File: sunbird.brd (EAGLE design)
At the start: 127 x 19.1 mm, 41 parts, among them J1 USB_MINI-B_SMT, Q1 600mA/40V, U1000 TP4056, U1500 FS312F-G, U1550 FS8205, U2000 MT3608, U4000 FM116B, U5000 CH340G, Y5000 12Mhz

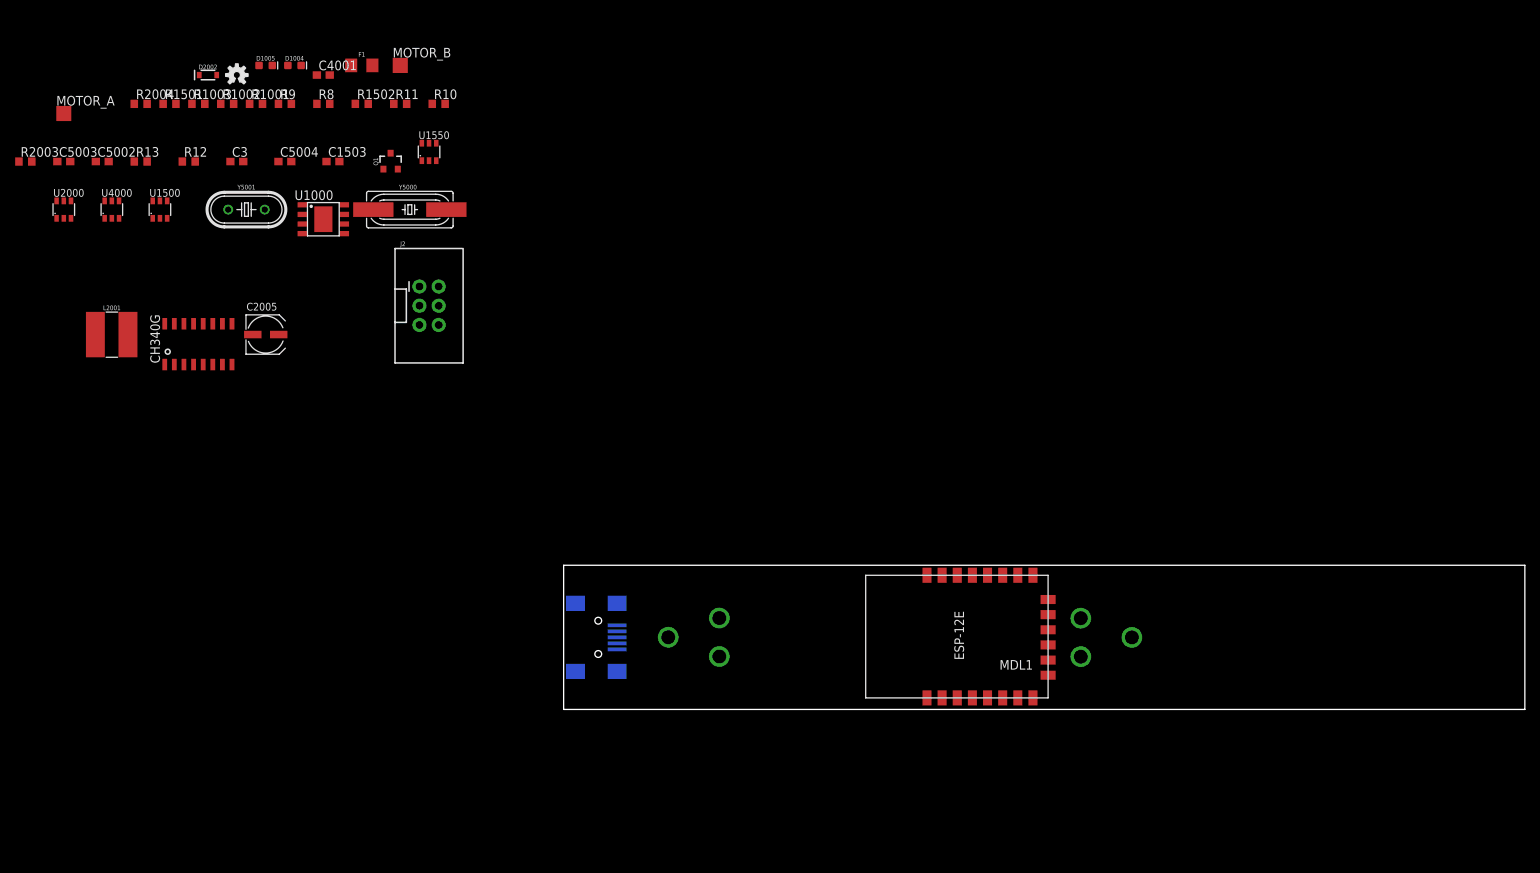
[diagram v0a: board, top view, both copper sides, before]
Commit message: Getting there
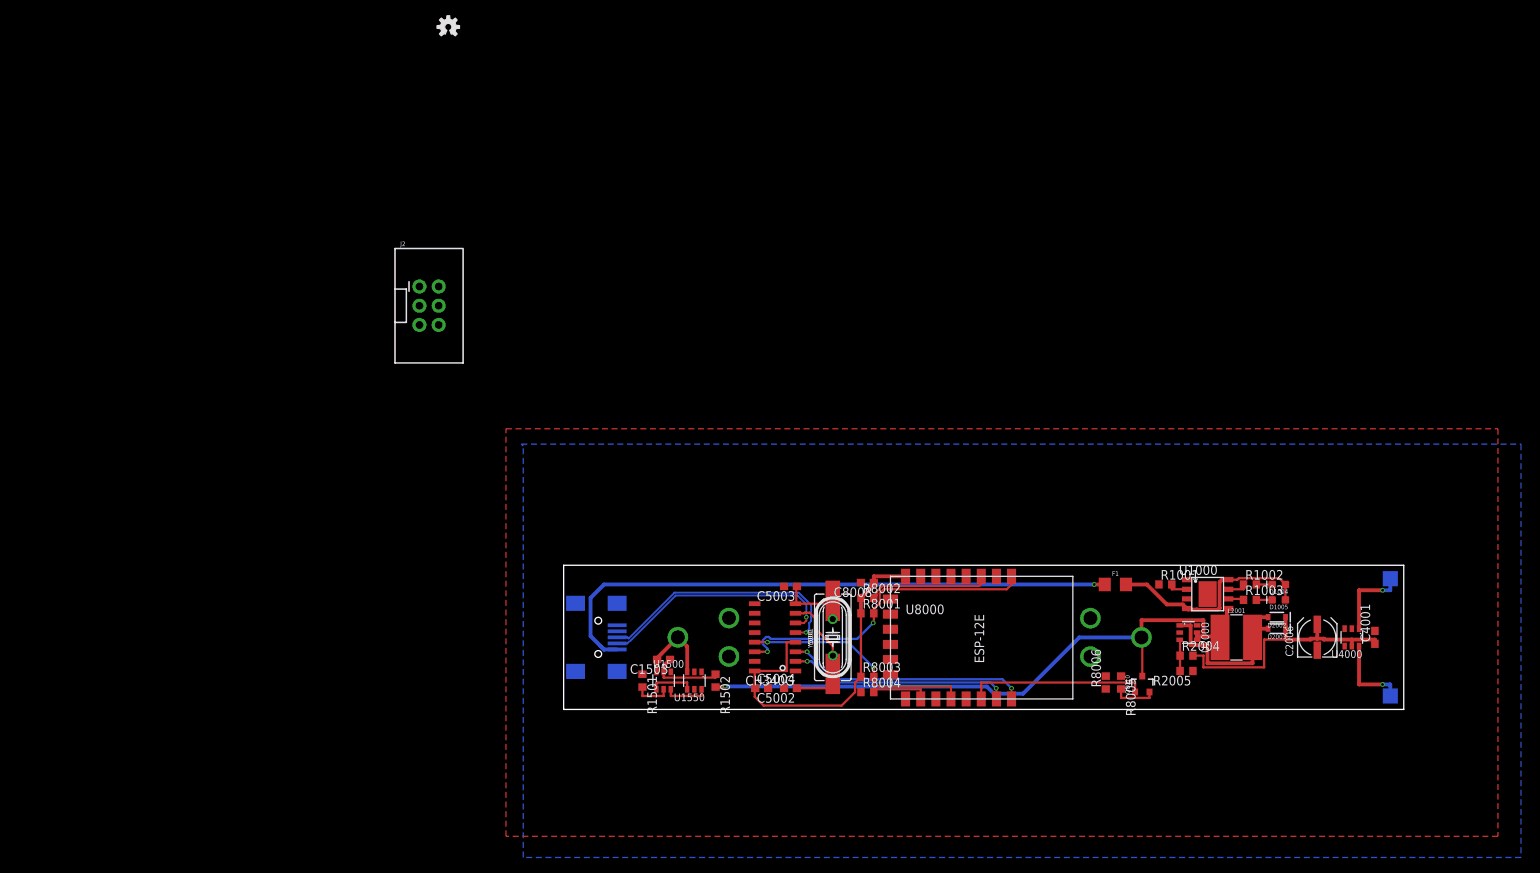
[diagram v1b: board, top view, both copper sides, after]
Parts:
- removed C2005: 47uF, rcl:UD-5X5,8_NICHICON
- removed C3: 0.1uf, rcl:C0603
- removed MDL1: (no value), ESP8266-ESP12E:ESP8266-ESP12E
- removed Q1: 600mA/40V, SparkFun-DiscreteSemi:SOT23-3
- removed R10, R11, R8, R9: 10k, rcl:R0603
- removed R12: 400k, rcl:R0603
- removed R13: 100k, rcl:R0603
- removed R2003: 4.5k, rcl:R0603
- added C2006: 47uF, rcl:UD-5X5,8_NICHICON
- added C8008: 0.1uf, rcl:C0603
- added D2003: (no value), SparkFun-DiscreteSemi:SOD-323
- added Q8010: 600mA/40V, SparkFun-DiscreteSemi:SOT23-3
- added R2005: 1k, rcl:R0603
- added R8001, R8002, R8003, R8004: 10k, rcl:R0603
- added R8005: 400k, rcl:R0603
- added R8006: 100k, rcl:R0603
- added U8000: (no value), ESP8266-ESP12E:ESP8266-ESP12E
- R2004: value 1k -> 4.5k
- moved MOTOR_A 191.4 mm to (109.2, 1.78), flipped to the bottom
- moved U4000 173.3 mm to (104.1, 9.53), turned to 180 degrees
- moved U2000 158.8 mm to (82.5, 10.2), turned to 270 degrees
- moved D2002 158.4 mm to (94.2, 12.2), turned to 180 degrees
- moved C4001 157.6 mm to (107.2, 9.53), turned to 90 degrees
- moved R2004 156.2 mm to (82.3, 7.11)
- moved L2001 153.9 mm to (88.9, 9.53)
- moved R1003 153.6 mm to (90.7, 14.5)
- moved D1005 151.3 mm to (94.5, 14.5), turned to 180 degrees
- moved R1002 149.3 mm to (90.7, 16.5)
- moved MOTOR_B 147.3 mm to (109.2, 17.3), flipped to the bottom
- moved D1004 147.0 mm to (94.5, 16.5), turned to 180 degrees
- moved R1001 135.9 mm to (79.5, 16.5)
- moved U1000 126.9 mm to (85.1, 15.2)
- moved F1 120.9 mm to (72.9, 16.5)
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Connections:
- net N$14 renamed MOTOR_A
- net N$15 renamed MOTOR_B
- removed net SCL: MDL1.14
- removed net SDA: MDL1.13
- removed net USB_D+: U5000.5
- removed net USB_D-: U5000.6
- new net GPIO4: U8000.13
- new net GPIO5: Q8010.1, U8000.14
- net 3.3V: now also C2006.+, C8008.1, D2003.C, R2004.2, R8001.1, R8002.1, R8003.1, U8000.8; no longer C2005.+, C3.1, MDL1.8, R10.1, R2003.2, R8.1, R9.1
- net ADC: now also R8005.1, R8006.2, U8000.2; no longer MDL1.2, R12.1, R13.2
- net CH_PD: now also R8002.2, U8000.3; no longer MDL1.3, R9.2
- net CS0: now also U8000.17; no longer MDL1.17
- net GND: now also C2006.-, C8008.2, R2005.1, R8004.1, R8006.1, U8000.9; no longer C2005.-, C3.2, MDL1.9, R11.1, R13.1, R2004.1
- net GPIO0: now also R8003.2, U8000.12; no longer MDL1.12, R10.2
- net GPIO10: now also U8000.20; no longer MDL1.20
- net GPIO12: now also U8000.6; no longer MDL1.6
- net GPIO13: now also U8000.7; no longer MDL1.7
- net GPIO14: now also U8000.5; no longer MDL1.5
- net GPIO15: now also R8004.2, U8000.10; no longer MDL1.10, R11.2
- net GPIO16: now also U8000.4; no longer MDL1.4, Q1.1
- net GPIO2: now also U8000.11; no longer MDL1.11
- net GPIO9: now also U8000.19; no longer MDL1.19
- net MISO: now also U8000.18; no longer MDL1.18
- net MOSI: now also U8000.21; no longer MDL1.21
- net N$12: now also D2003.A
- net N$13: now also R2004.1, R2005.2; no longer R2003.1, R2004.2
- net N$9: now also Q8010.2, R8005.2; no longer Q1.2, R12.2
- net RESET: now also R8001.2, U8000.1; no longer MDL1.1, R8.2
- net RX: now also U8000.15; no longer MDL1.15
- net SCLK: now also U8000.22; no longer MDL1.22
- net TX: now also U8000.16; no longer MDL1.16
- net USB_N: now also U5000.6
- net USB_P: now also U5000.5
- net V_BATT: now also Q8010.3; no longer Q1.3
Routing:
- net V_BATT: track 0.00 -> 86.6 mm, vias 0 -> 1
- net 3.3V: track 0.00 -> 83.5 mm
- net N$17: track 0.00 -> 78.7 mm, vias 0 -> 1
- net RESET: track 0.00 -> 42.4 mm, vias 0 -> 2
- net USB_P: track 0.00 -> 34.2 mm, vias 0 -> 1
- net TX: track 0.00 -> 32.0 mm, vias 0 -> 2
- net USB_N: track 0.00 -> 31.6 mm, vias 0 -> 1
- net GPIO0: track 0.00 -> 31.4 mm, vias 0 -> 2
- net RX: track 0.00 -> 29.4 mm, vias 0 -> 2
- net V_USB: track 0.00 -> 28.6 mm
- net N$12: track 0.00 -> 25.5 mm
- net GPIO5: track 0.00 -> 23.7 mm
- net OSCI: track 0.00 -> 18.3 mm
- net CH_PD: track 0.00 -> 16.2 mm
- net N$5: track 0.00 -> 10.8 mm
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- added copper zone on layer 1, net GND
- added copper zone on layer 16, net GND
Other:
- board size 127 x 19.1 mm -> 111 x 19.1 mm
